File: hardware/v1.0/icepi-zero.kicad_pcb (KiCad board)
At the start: 4 copper layers, 65 x 30 mm, 138 parts, among them J1 Conn_02x20_Counter_Clockwise, J2 HDMI_C_1.3, J3 USB_C_Receptacle_USB2.0_14P, J4 USB_C_Receptacle_USB2.0_14P, J5 USB_C_Receptacle_USB2.0_14P, J6 Micro_SD_Card_Det2, SW1 SW_Push, U1 ECP5U_12_CABGA256, U10 W9825G6KH, U11 W25Q128JVS, U2 TLV62569DBV, U3 TLV62569DBV, U4 TLV62569DBV, U5 PCA9306DC1, U6 FT231XQ, U7 TPD2EUSB30A, U8 TPD2EUSB30A, U9 TPD2EUSB30A, Y1 SITxxxxxx-1x-33E-50.000000

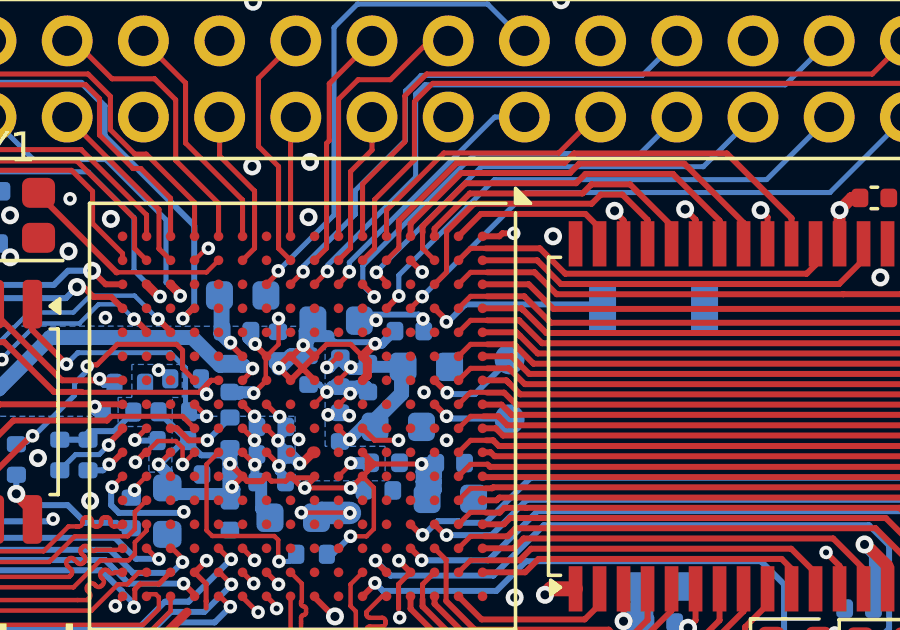
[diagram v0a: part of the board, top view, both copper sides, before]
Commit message: Counter example start - button on off
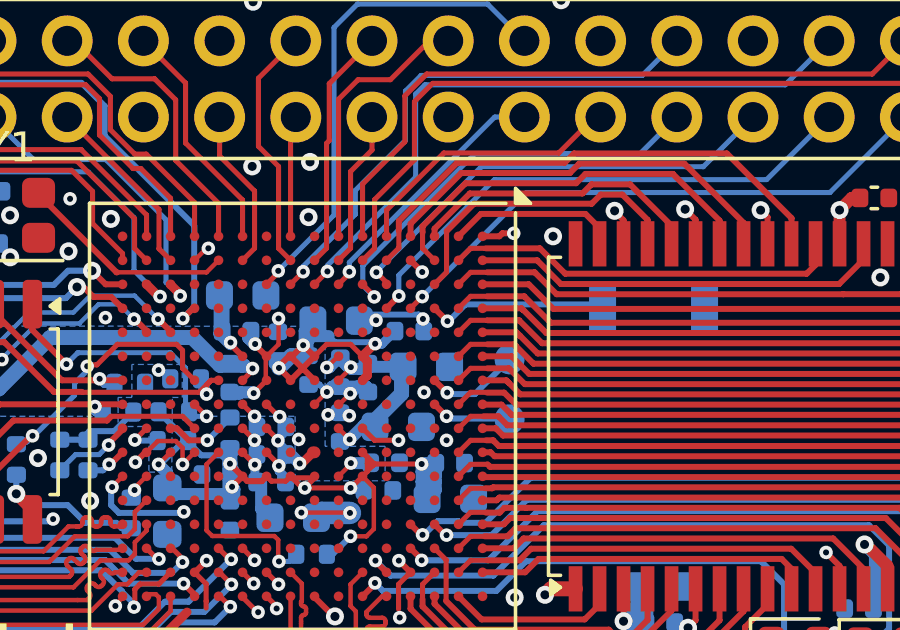
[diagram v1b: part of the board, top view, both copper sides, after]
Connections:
- U1 pad C5: SW2 -> unconnected-(U1B-PT15A/+-PadC5)
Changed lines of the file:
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@@
 	(net 248 "unconnected-(U1G-PL17D{slash}-{slash}LDQ20-PadJ5)")
 	(net 249 "unconnected-(U1E-PR29D{slash}-{slash}RDQ32-PadL12)")
-	(net 250 "SW2")
+	(net 250 "unconnected-(U1B-PT15A{slash}+-PadC5)")
 	(footprint "MountingHole:MountingHole_2.7mm_M2.5"
 		(layer "F.Cu")
@@
 			(property pad_prop_bga)
 			(layers "F.Cu" "F.Mask" "F.Paste")
-			(net 250 "SW2")
+			(net 250 "unconnected-(U1B-PT15A{slash}+-PadC5)")
 			(pinfunction "PT15A/+")
-			(pintype "bidirectional")
+			(pintype "bidirectional+no_connect")
 		)
 		(pad "C6" smd circle
@@
 	)
 	(segment
-		(start 154.791822 101.541822)
+		(start 154.828767 101.578767)
 		(end 154.4 101.15)
 		(width 0.2)
@@
 	)
 	(segment
-		(start 154.791822 101.600568)
-		(end 154.791822 101.541822)
+		(start 154.754877 101.578767)
+		(end 154.749432 101.584212)
+		(width 0.2)
+		(layer "F.Cu")
+		(net 160)
+	)
+	(segment
+		(start 154.749432 101.584212)
+		(end 154.749432 101.600568)
+		(width 0.2)
+		(layer "F.Cu")
+		(net 160)
+	)
+	(segment
+		(start 154.828767 101.578767)
+		(end 154.754877 101.578767)
 		(width 0.2)
 		(layer "F.Cu")
@@
 	)
 	(via
-		(at 154.791822 101.600568)
+		(at 154.828767 101.578767)
 		(size 0.45)
 		(drill 0.2)
@@
 	)
 	(segment
+		(start 159.87 101.02)
+		(end 160 101.15)
+		(width 0.2)
+		(layer "B.Cu")
+		(net 160)
+	)
+	(segment
 		(start 155.43 101.02)
 		(end 159.87 101.02)
@@
 	)
 	(segment
-		(start 159.87 101.02)
-		(end 160 101.15)
+		(start 154.865712 101.541822)
+		(end 154.908178 101.541822)
 		(width 0.2)
 		(layer "B.Cu")
@@
 	)
 	(segment
-		(start 154.849432 101.600568)
+		(start 154.908178 101.541822)
 		(end 155.43 101.02)
 		(width 0.2)
@@
 	)
 	(segment
-		(start 154.791822 101.600568)
-		(end 154.849432 101.600568)
+		(start 154.828767 101.578767)
+		(end 154.865712 101.541822)
 		(width 0.2)
 		(layer "B.Cu")
